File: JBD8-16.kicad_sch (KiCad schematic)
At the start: 64 parts, among them J1 RS232, J2 5V, SW1 RESET, U1 74LS02, U1 W65C02SxP, U11 74LS21, U12 74LS04, U13 74LS21, U14 74LS86, U15 74LS08, U16 74LS27, U17 74LS21, U18 74LS02, U19 74LS32, U2 74LS11, U20 74LS08, U21 74LS154, U22 74LS21, U23 74LS154, U24 74LS30, U25 74LS30, U26 74LS08, U27 74LS04, U28 74LS154, U29 74LS30, U3 28C256(ROM), U30 CY62256-70PC(RAM), U31 CY62256-70PC(RAM), U32 CY62256-70PC(RAM), U33 CY62256-70PC(RAM), U34 CY62256-70PC(RAM), U35 CY62256-70PC(RAM), U36 CY62256-70PC(RAM), U4 74LS04, U4 CY62256-70PC(RAM), U46 74LS245, U5 74LS04, U5 W65C51NxP, U6 74LS11, U6 MAX232, U7 74LS154, U8 74LS373, U9 74LS138, X1 1Mhz, Y1 1.8432Mhz

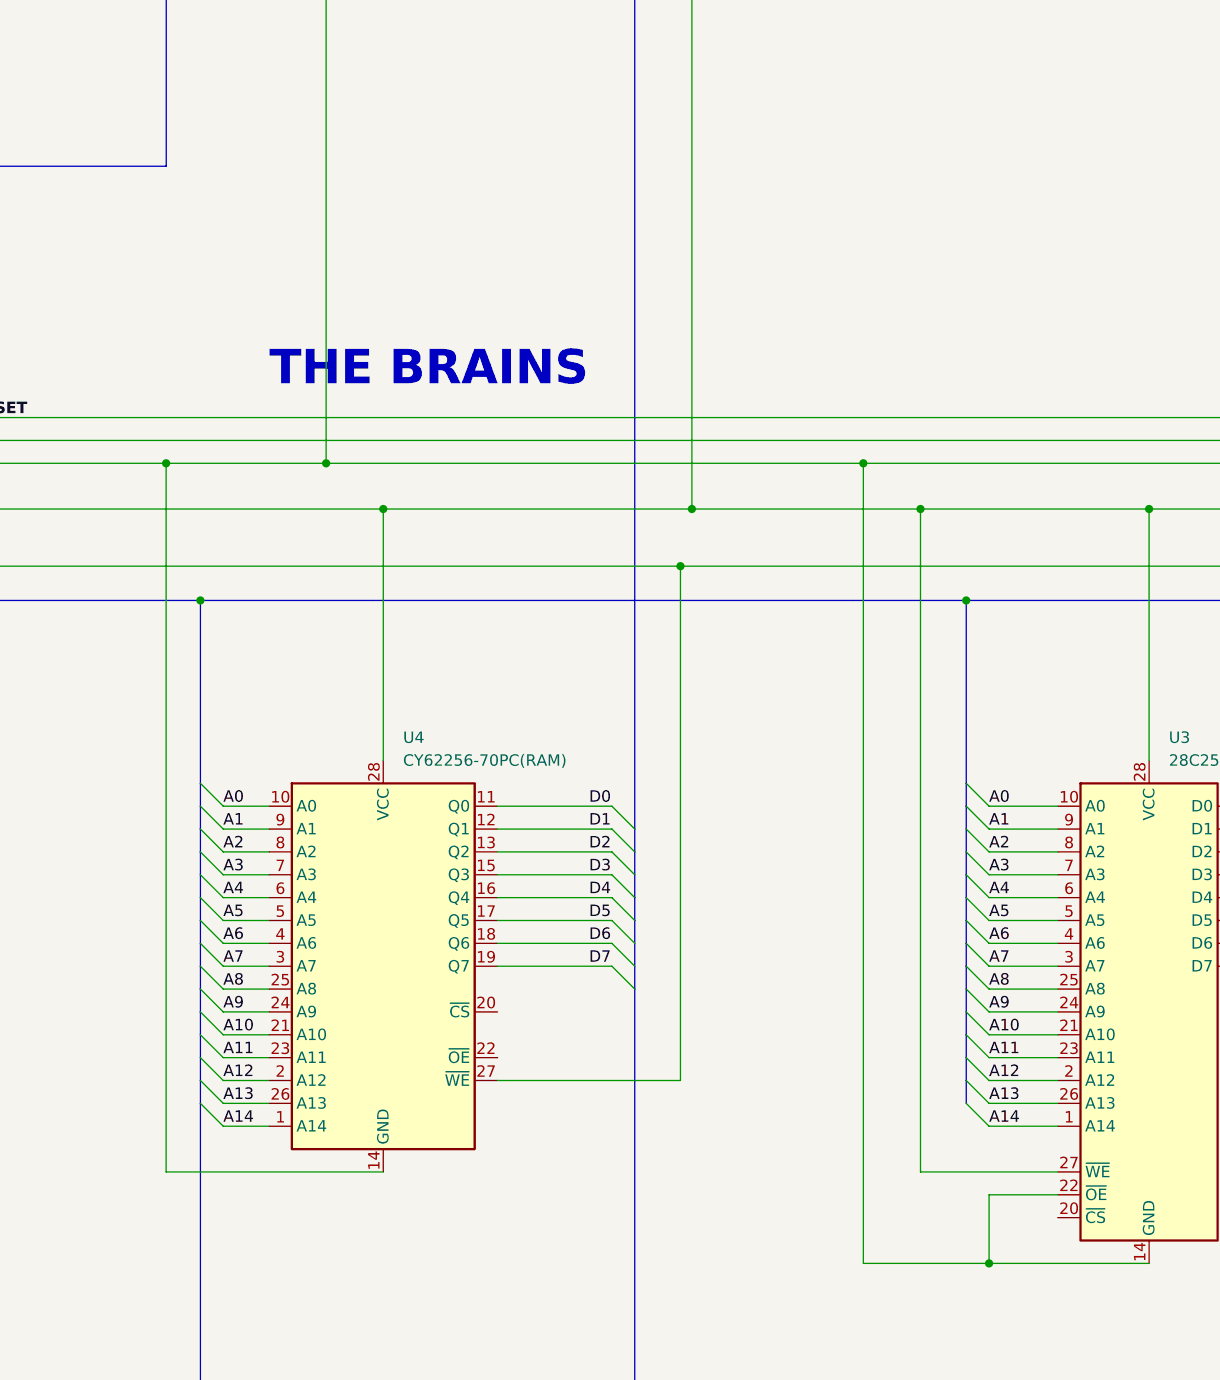
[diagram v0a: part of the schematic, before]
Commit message: worked on the CS on some chips
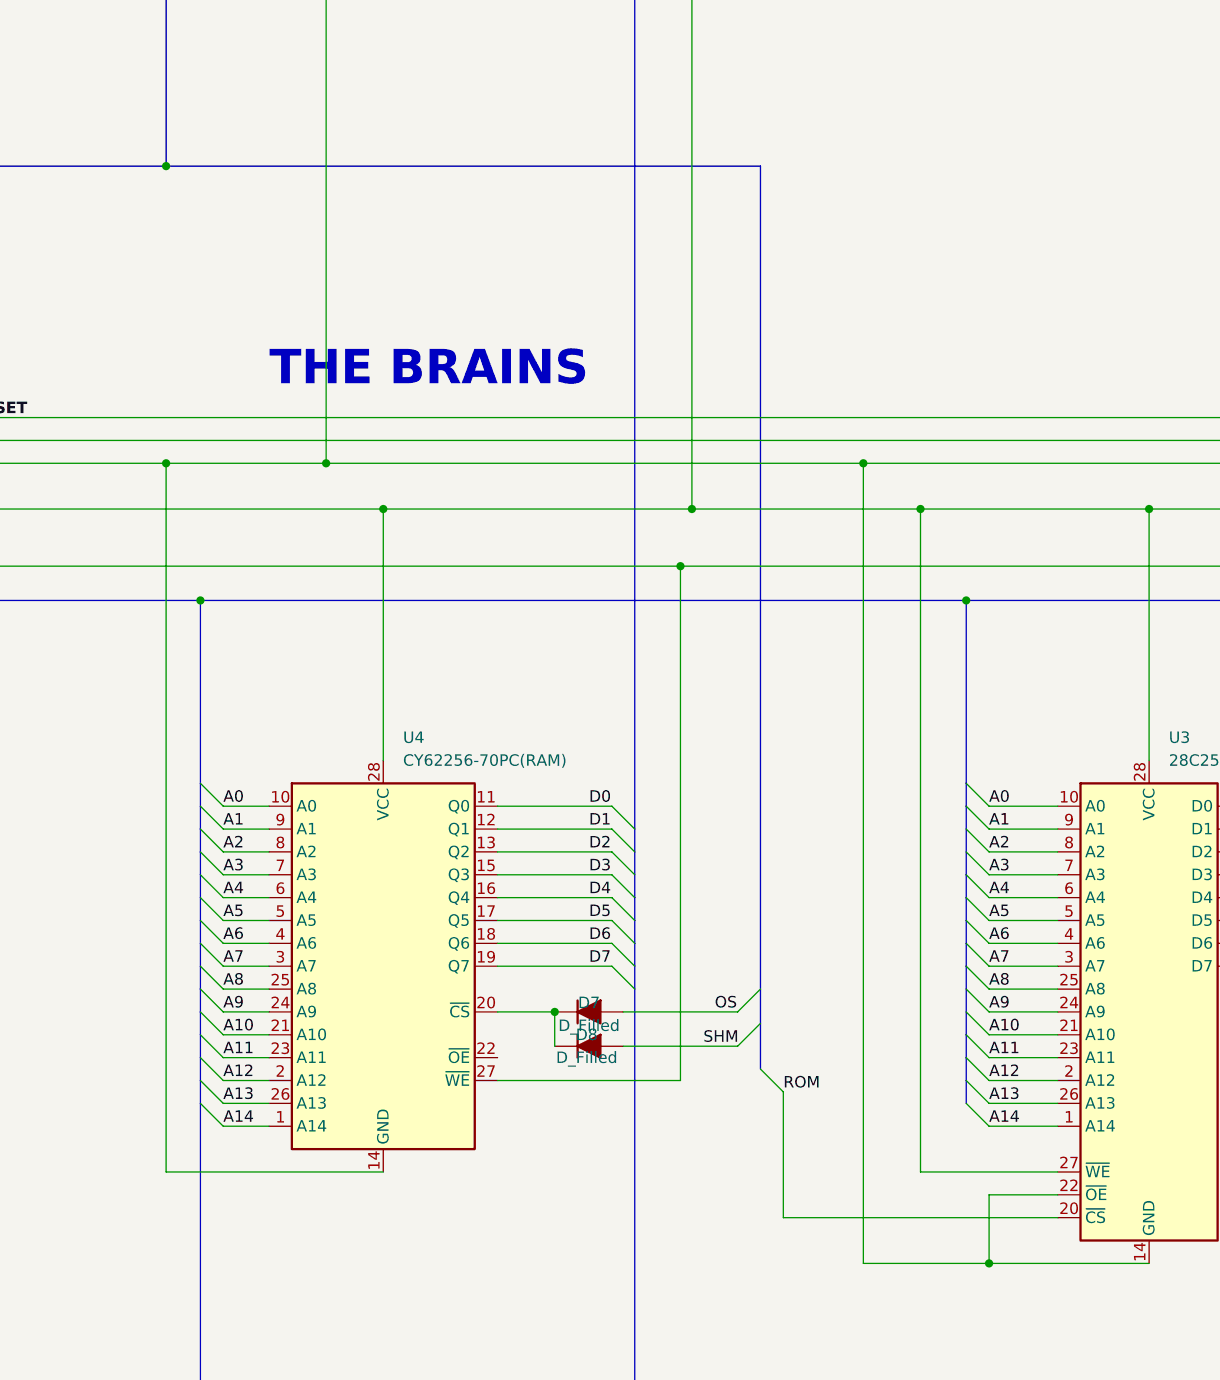
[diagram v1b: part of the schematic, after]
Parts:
- added D7, D8: D_Filled, symbol Device:D_Filled
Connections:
- net OS: now also D7.2 (A)
- net ROM: now also U3.20 (~{CS})
- net SHM: now also D8.2 (A)
- net at U4.20 (~{CS}): now also D7.1 (K), D8.1 (K)
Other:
- title: BE6502+ -> JBD8-8
